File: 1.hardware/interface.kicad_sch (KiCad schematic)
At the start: 37 parts, among them J12 ESP_DM_COMM, J13 ESP_DP_COMM, J14 ESP_DBG, J15 Can_conn, J16 Conn_01x04, J7 uart_comm, J8 USB_C, J9 ESP_BOOT_CONN, U11 SN65HVD230, U5 ESP32-C3-WROOM-02

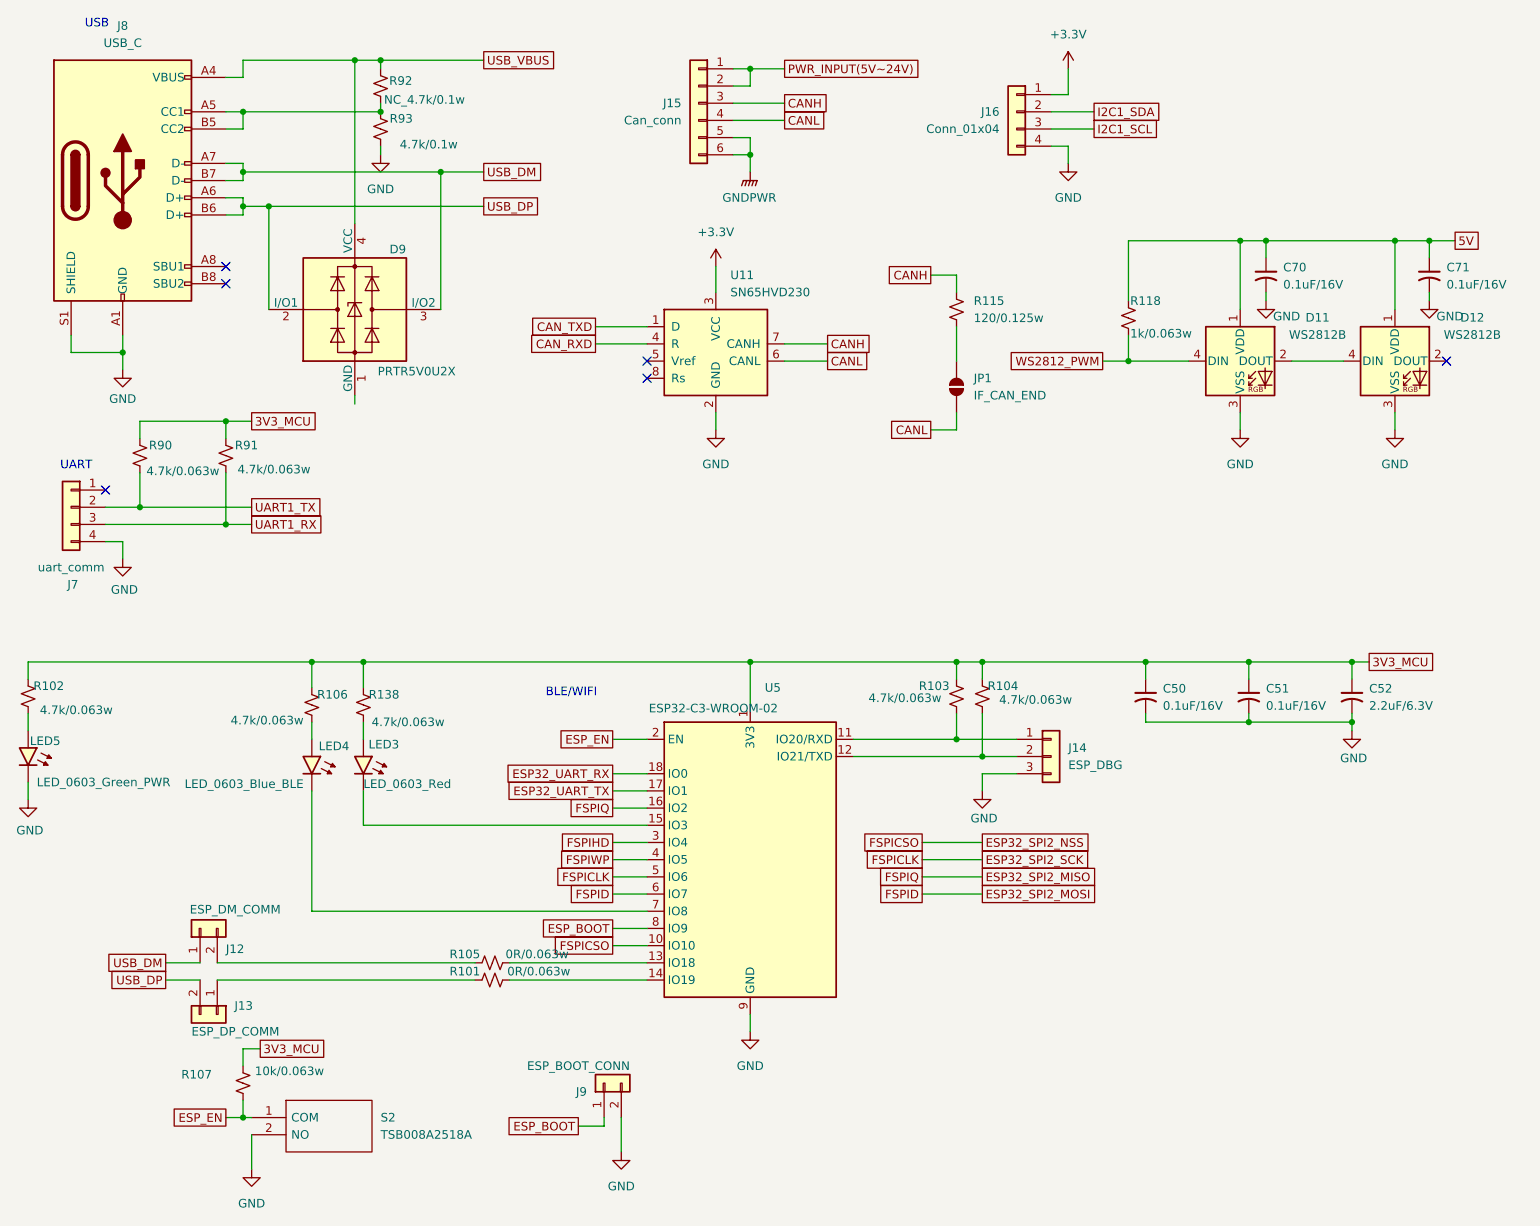
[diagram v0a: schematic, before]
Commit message: 중간 저장
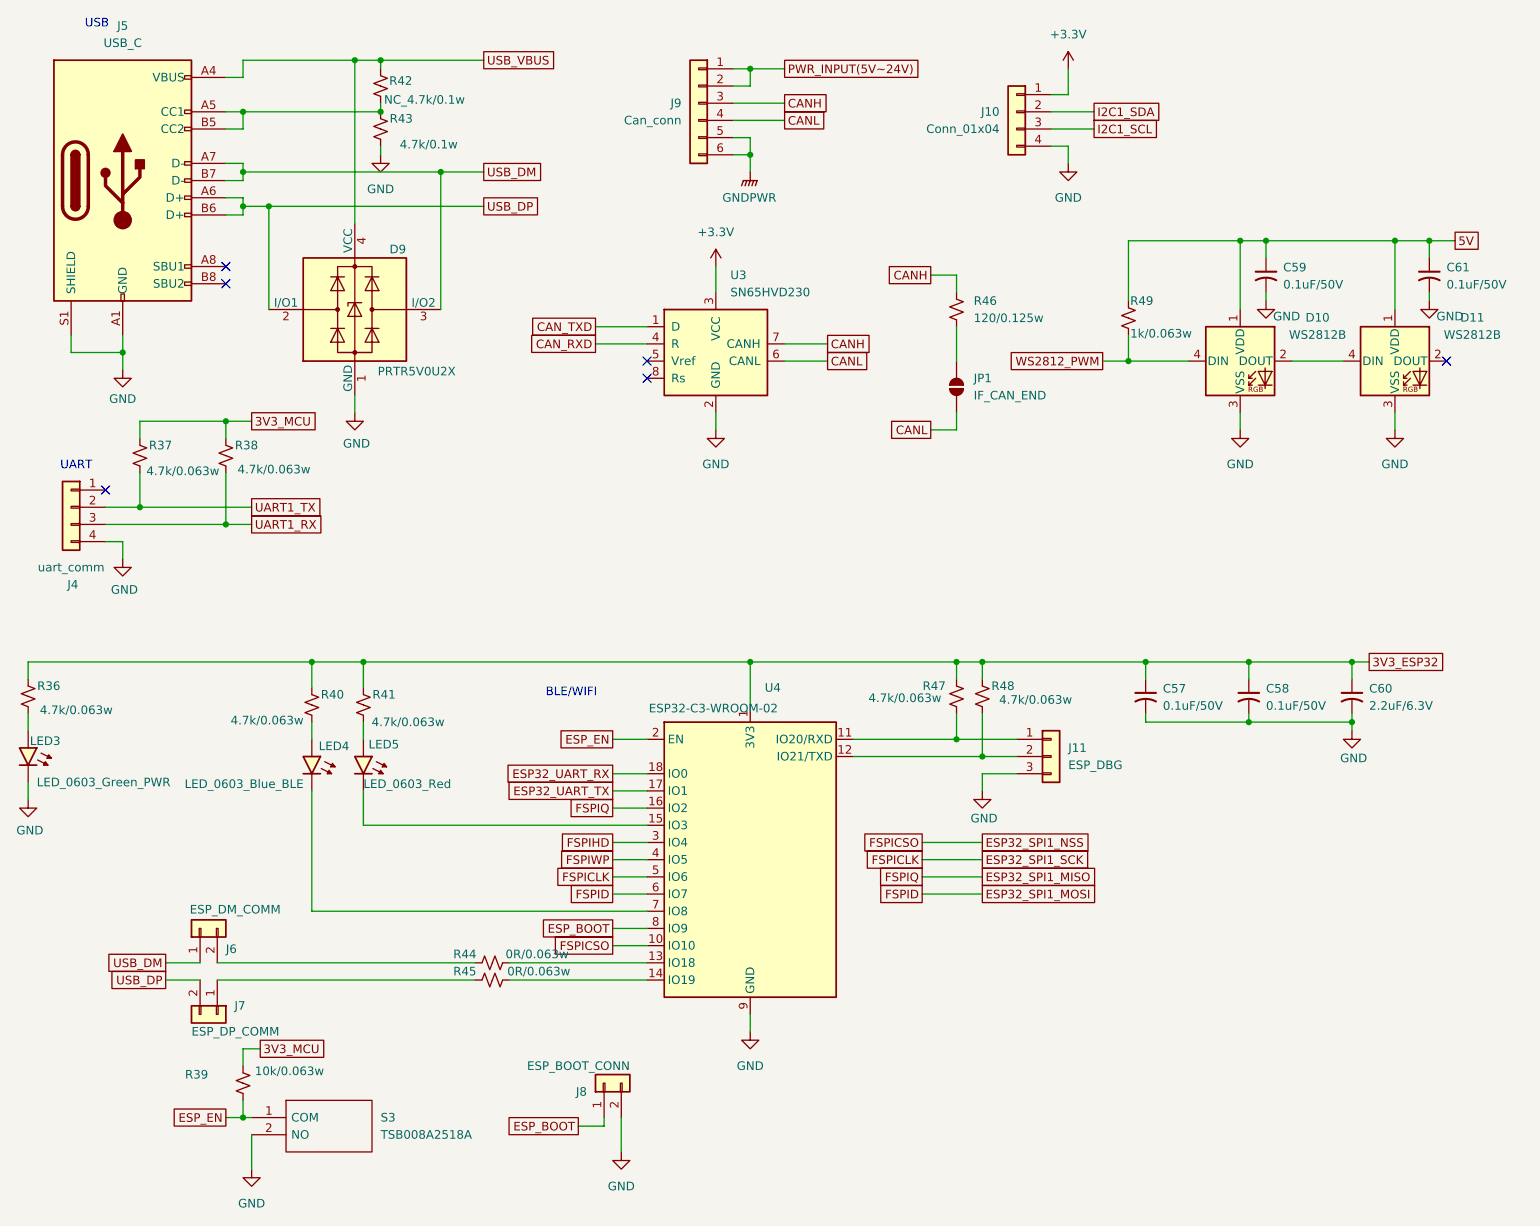
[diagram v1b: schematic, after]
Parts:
- C57: renamed from C50; value 0.1uF/16V -> 0.1uF/50V; footprint Capacitor_SMD:C_0402_1005Metric -> Capacitor_SMD:C_0603_1608Metric
- C58: renamed from C51; value 0.1uF/16V -> 0.1uF/50V; footprint Capacitor_SMD:C_0402_1005Metric -> Capacitor_SMD:C_0603_1608Metric
- C59: renamed from C70; value 0.1uF/16V -> 0.1uF/50V; footprint Capacitor_SMD:C_0402_1005Metric -> Capacitor_SMD:C_0603_1608Metric
- C61: renamed from C71; value 0.1uF/16V -> 0.1uF/50V; footprint Capacitor_SMD:C_0402_1005Metric -> Capacitor_SMD:C_0603_1608Metric
- R39: renamed from R107; footprint (none) -> Resistor_SMD:R_0402_1005Metric
- R44: renamed from R105; footprint (none) -> Resistor_SMD:R_0402_1005Metric
- R45: renamed from R101; footprint (none) -> Resistor_SMD:R_0402_1005Metric
- R46: renamed from R115; footprint (none) -> Resistor_SMD:R_0805_2012Metric
- R49: renamed from R118; footprint (none) -> Resistor_SMD:R_0402_1005Metric
- renumbered C52 to C60, D11 to D10, D12 to D11, J16 to J10, J14 to J11, J7 to J4, J8 to J5, J12 to J6, J13 to J7, J9 to J8, J15 to J9, LED5 to LED3, LED3 to LED5, R102 to R36, R90 to R37, R91 to R38, R106 to R40, R138 to R41, R92 to R42, R93 to R43, R103 to R47, R104 to R48, S2 to S3, U11 to U3, U5 to U4
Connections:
- net 3V3_MCU: no longer C57.1, C58.1, C60.1, R36.1, R40.1, R41.1, R47.1, R48.1, U4.1 (3V3)
- net GND: now also D9.1 (GND)
- net ESP32_SPI2_MISO renamed ESP32_SPI1_MISO
- net ESP32_SPI2_MOSI renamed ESP32_SPI1_MOSI
- net ESP32_SPI2_NSS renamed ESP32_SPI1_NSS
- net ESP32_SPI2_SCK renamed ESP32_SPI1_SCK
- new net 3V3_ESP32: C57.1, C58.1, C60.1, R36.1, R40.1, R41.1, R47.1, R48.1, U4.1 (3V3)

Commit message: 중간 저장
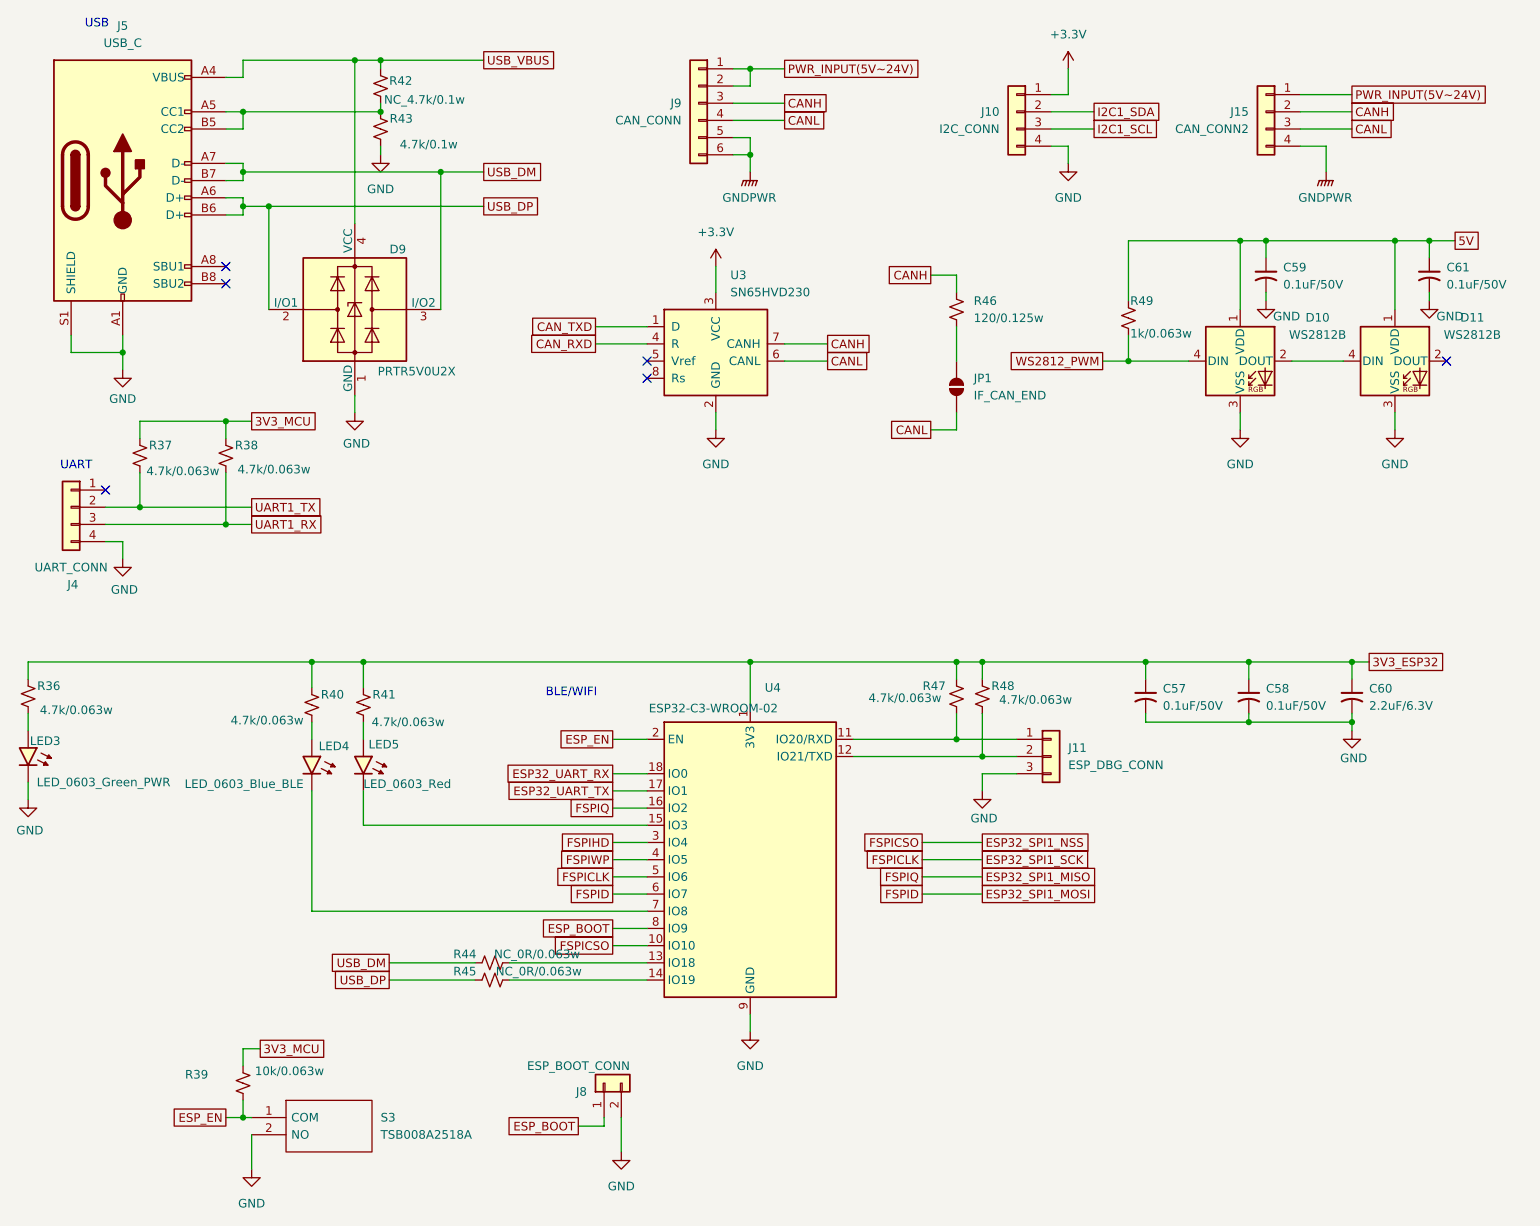
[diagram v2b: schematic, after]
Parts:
- removed J6: ESP_DM_COMM, symbol Connector_Generic:Conn_01x02
- removed J7: ESP_DP_COMM, symbol Connector_Generic:Conn_01x02
- added J15: CAN_CONN2, symbol Connector_Generic:Conn_01x04
- J10: value Conn_01x04 -> I2C_CONN
- J11: value ESP_DBG -> ESP_DBG_CONN
- J4: value uart_comm -> UART_CONN
- J9: value Can_conn -> CAN_CONN
- R44, R45: value 0R/0.063w -> NC_0R/0.063w
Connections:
- net CANH: now also J15.2 (Pin_2)
- net CANL: now also J15.3 (Pin_3)
- net GNDPWR: now also J15.4 (Pin_4)
- net PWR_INPUT(5V~24V): now also J15.1 (Pin_1)
- net USB_DM: now also R44.1
- net USB_DP: now also R45.1
